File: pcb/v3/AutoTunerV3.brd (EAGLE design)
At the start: 100 x 80 mm, 115 parts, among them IC2 317EMP, Q1 32,768kHz, Q2 BSS123, Q3 BSS84, U1 TPS63070RNMR, Y1 8MHz

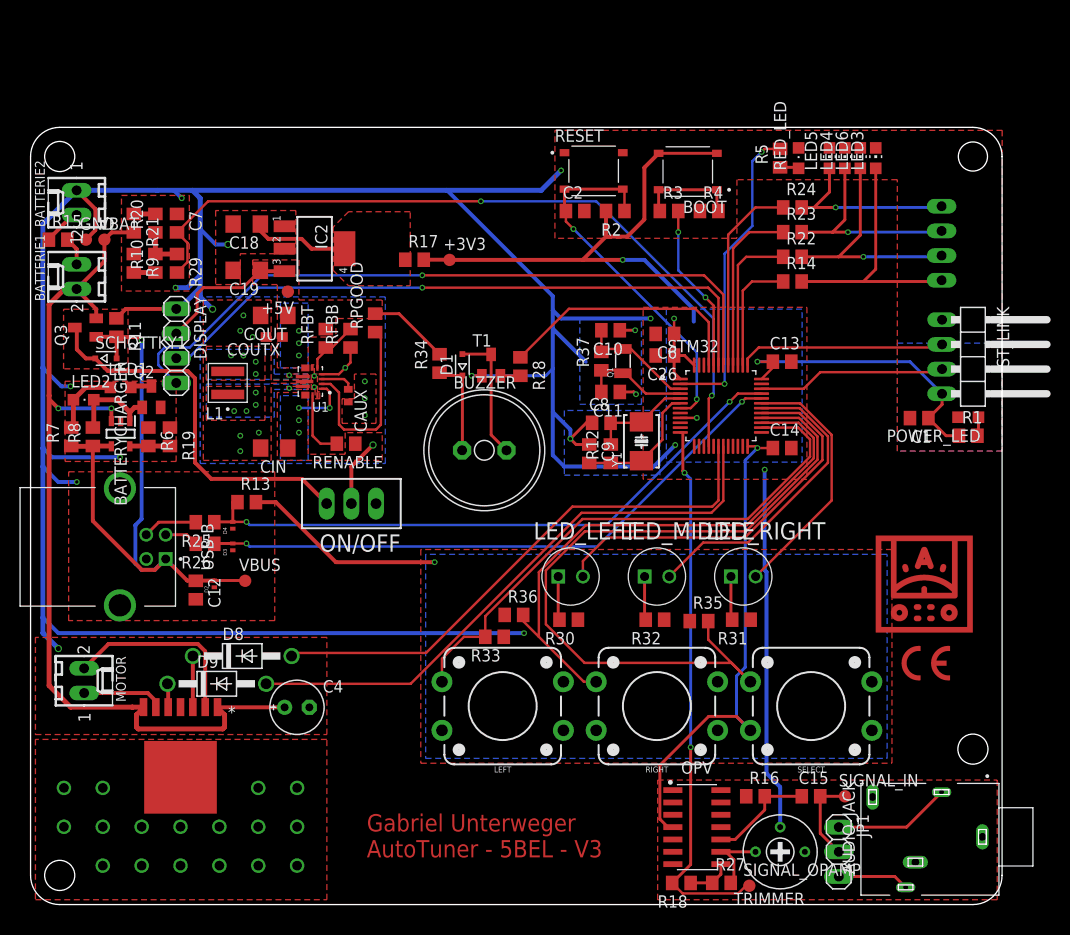
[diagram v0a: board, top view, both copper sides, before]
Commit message: board v3 finished
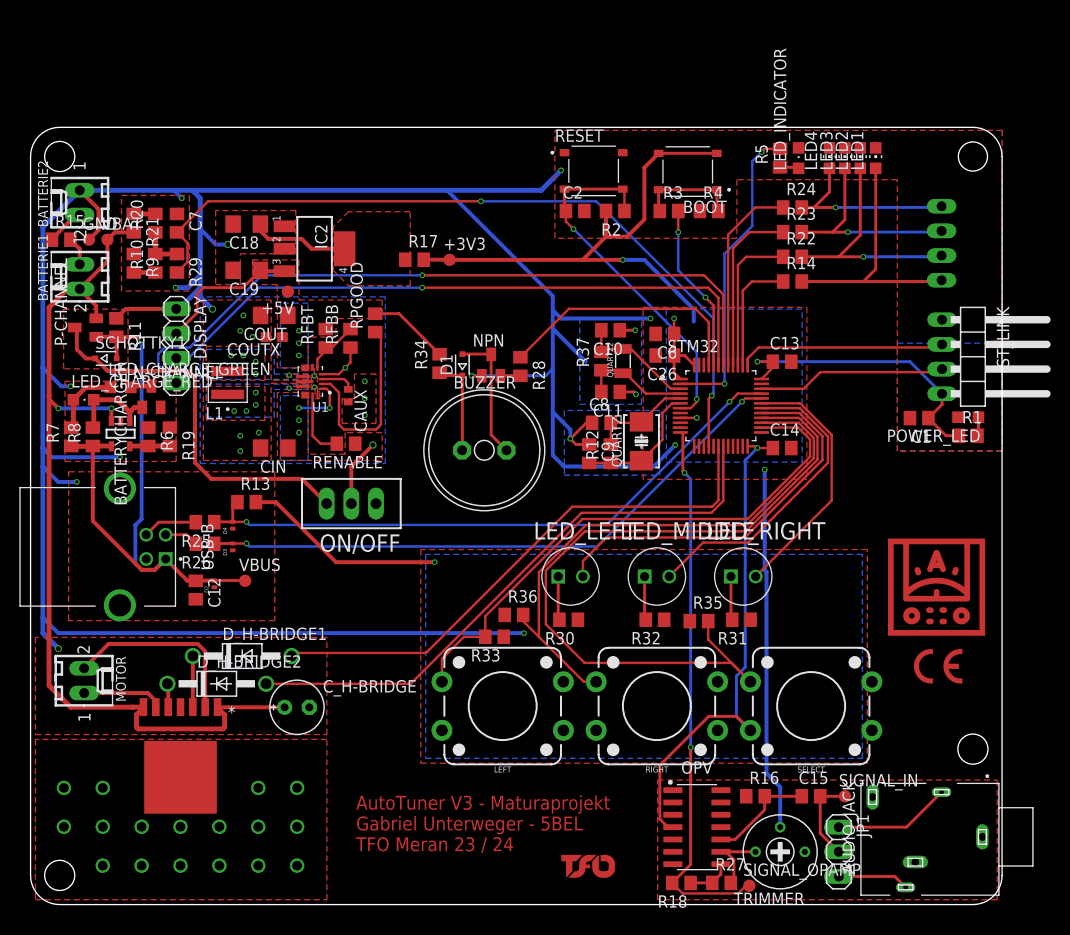
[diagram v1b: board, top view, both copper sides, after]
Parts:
- removed LED5, LED6: (no value), led:CHIP-LED0805
- added LED_CHARGE_GREEN, LED_CHARGE_RED: (no value), led:CHIPLED_0805
- LED1, LED2: device led:CHIPLED_0805 -> led:CHIP-LED0805
- R32: value 60 -> 56
- moved LED2 83.7 mm to (85.4, 76.8), turned to 0 degrees
- moved LED1 81.2 mm to (87.0, 76.8), turned to 0 degrees
- moved LED3 3.18 mm to (83.8, 76.8)
- moved LED4 1.59 mm to (82.2, 76.8)
- moved VBAT 0.32 mm to (7.92, 68.4)
- moved BATTERIE1 0.32 mm to (5.06, 64.6)
- moved BATTERIE2 0.32 mm to (5.06, 72.2)
- moved GND 0.32 mm to (6.01, 68.4)
- moved R15 0.32 mm to (3.15, 68.4)
- renumbered C4 to C_H-BRIDGE, D8 to D_H-BRIDGE1, D9 to D_H-BRIDGE2, JP2 to EXTENSIONS, Q1 to QUARTZ2, Q2 to N-CHANNEL, Q3 to P-CHANNEL, RED_LED to LED_INDICATOR, T1 to NPN, Y1 to QUARTZ
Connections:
- net GND: now also LED1.C, LED2.C; no longer LED5.C, LED6.C
- net N$11: now also LED_CHARGE_GREEN.A, LED_CHARGE_RED.A; no longer LED1.A, LED2.A
- net N$12: now also LED_CHARGE_GREEN.C; no longer LED1.C
- net N$39: now also LED1.A; no longer LED3.A
- net N$48: now also LED2.A; no longer LED6.A
- net N$49: now also LED3.A; no longer LED4.A
- net N$50: now also LED4.A; no longer LED5.A
- net N$9: now also LED_CHARGE_RED.C; no longer LED2.C
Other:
- board text added: "AutoTuner V3 - Maturaprojekt Gabriel Unterweger - 5BEL TFO Meran 23 / 24"
- board text removed: "Gabriel Unterweger AutoTuner - 5BEL - V3"

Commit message: settings menu
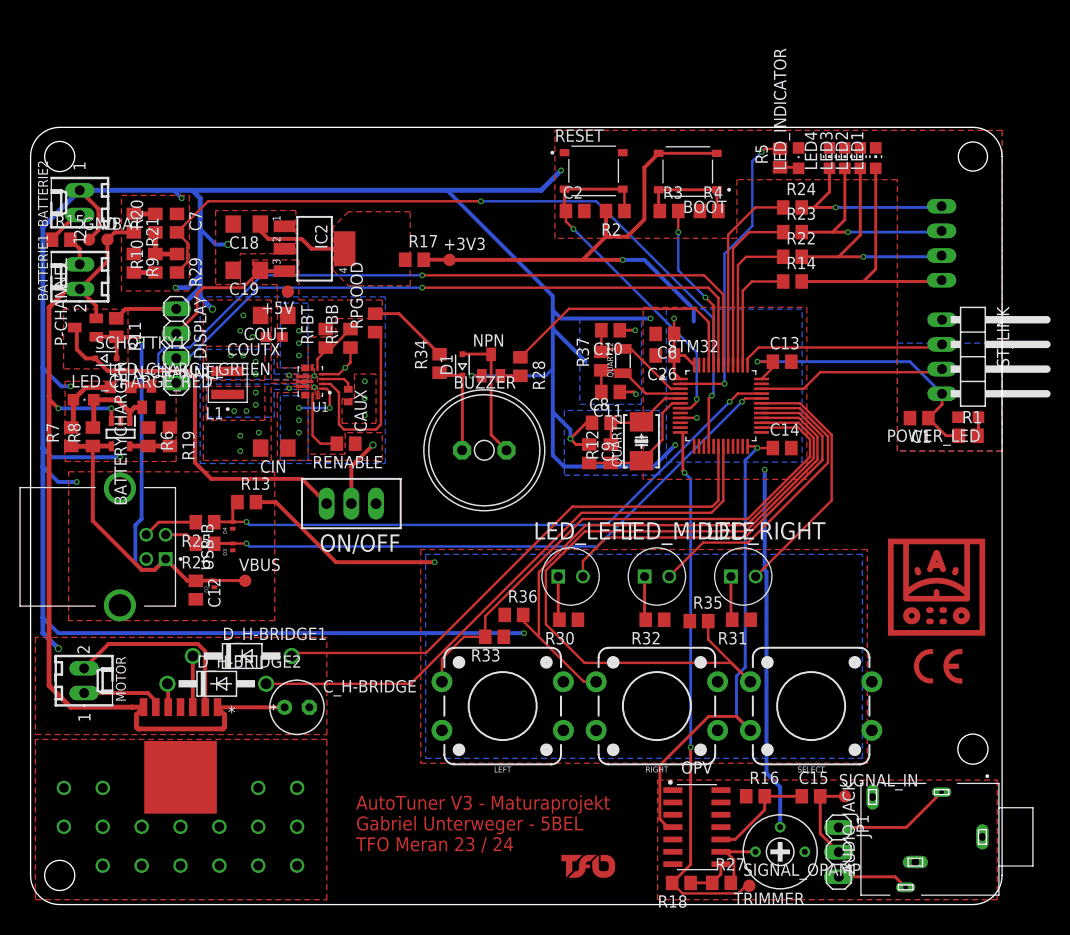
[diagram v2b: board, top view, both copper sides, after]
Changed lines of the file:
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@@
 <drawing>
 <settings>
-<setting alwaysvectorfont="yes"/>
+<setting alwaysvectorfont="no"/>
 <setting verticaltext="up"/>
 </settings>
@@
 <attribute name="VALUE" x="79.675" y="11.035" size="1.27" layer="27" rot="R180"/>
 </element>
-<element name="JP1" library="pinhead" library_urn="urn:adsk.eagle:library:325" package="1X03" package3d_urn="urn:adsk.eagle:package:22458/2" value="" x="83.1925" y="5.43" smashed="yes" rot="R270">
-<attribute name="NAME" x="85.0213" y="9.3162" size="1.27" layer="25" ratio="10" rot="R270"/>
-<attribute name="POPULARITY" value="92" x="83.1925" y="5.43" size="1.778" layer="27" rot="R270" display="off"/>
-<attribute name="VALUE" x="80.0175" y="9.24" size="1.27" layer="27" rot="R270"/>
-</element>
 <element name="LED1" library="led" library_urn="urn:adsk.eagle:library:259" package="CHIP-LED0805" package3d_urn="urn:adsk.eagle:package:15818/2" value="" x="86.995" y="76.835" smashed="yes">
 <attribute name="LCSC_PART" value="C2297" x="86.995" y="76.835" size="1.778" layer="27" display="off"/>
@@
 <attribute name="VALUE" x="25.7175" y="60.325" size="1.27" layer="27" rot="R180"/>
 </element>
+<element name="JP1" library="pinhead" library_urn="urn:adsk.eagle:library:325" package="1X03" package3d_urn="urn:adsk.eagle:package:22458/2" value="" x="83.185" y="5.3975" smashed="yes" rot="R270">
+<attribute name="NAME" x="85.0138" y="9.2837" size="1.27" layer="25" ratio="10" rot="R270"/>
+<attribute name="POPULARITY" value="92" x="83.185" y="5.3975" size="1.778" layer="27" rot="R270" display="off"/>
+<attribute name="VALUE" x="80.01" y="9.2075" size="1.27" layer="27" rot="R270"/>
+</element>
 </elements>
 <signals>
@@
 <signal name="N$11">
 <contactref element="LED_CHARGE_GREEN" pad="A"/>
-<contactref element="LED_CHARGE_RED" pad="A"/>
 <contactref element="R7" pad="2"/>
-<wire x1="4.1875" y1="49.1" x2="4.4075" y2="49.32" width="0.508" layer="1"/>
+<wire x1="8.2175" y1="53.23" x2="5.6775" y2="53.23" width="0.508" layer="1"/>
+<contactref element="LED_CHARGE_RED" pad="A"/>
+<wire x1="5.6775" y1="53.23" x2="4.4075" y2="51.96" width="0.508" layer="1"/>
 <wire x1="4.4075" y1="51.96" x2="4.4075" y2="49.32" width="0.508" layer="1"/>
-<wire x1="4.4075" y1="51.96" x2="5.6775" y2="53.23" width="0.508" layer="1"/>
-<wire x1="5.6775" y1="53.23" x2="8.2175" y2="53.23" width="0.508" layer="1"/>
+<wire x1="4.4075" y1="49.32" x2="4.1875" y2="49.1" width="0.508" layer="1"/>
 </signal>
 <signal name="N$9">
@@
 <contactref element="AUDIO_JACK" pad="5"/>
 <contactref element="JP1" pad="1"/>
-<wire x1="93.775" y1="11.57" x2="90.175" y2="7.97" width="0.3048" layer="1"/>
-<wire x1="90.175" y1="7.97" x2="83.1925" y2="7.97" width="0.3048" layer="1"/>
+<wire x1="90.1425" y1="7.9375" x2="83.185" y2="7.9375" width="0.3048" layer="1"/>
+<wire x1="93.775" y1="11.57" x2="90.1425" y2="7.9375" width="0.3048" layer="1"/>
 </signal>
 <signal name="SIGNAL_IN_2">
 <contactref element="AUDIO_JACK" pad="2"/>
 <contactref element="JP1" pad="3"/>
-<wire x1="83.1925" y1="2.89" x2="88.955" y2="2.89" width="0.3048" layer="1"/>
-<wire x1="88.955" y1="2.89" x2="90.075" y2="1.77" width="0.3048" layer="1"/>
+<wire x1="90.075" y1="1.77" x2="88.9875" y2="2.8575" width="0.3048" layer="1"/>
+<wire x1="88.9875" y1="2.8575" x2="83.185" y2="2.8575" width="0.3048" layer="1"/>
 </signal>
 <signal name="SIGNAL_IN">
-<contactref element="JP1" pad="2"/>
 <contactref element="C15" pad="2"/>
 <contactref element="SIGNAL_IN" pad="TP"/>
-<wire x1="83.1925" y1="5.43" x2="81.285" y2="7.3375" width="0.3048" layer="1"/>
-<wire x1="81.285" y1="7.3375" x2="81.285" y2="11.145" width="0.3048" layer="1"/>
 <wire x1="83.8275" y1="11.145" x2="81.285" y2="11.145" width="0.3048" layer="1"/>
+<contactref element="JP1" pad="2"/>
+<wire x1="83.185" y1="5.3975" x2="81.285" y2="7.2975" width="0.3048" layer="1"/>
+<wire x1="81.285" y1="7.2975" x2="81.285" y2="11.145" width="0.3048" layer="1"/>
 </signal>
 <signal name="CUSTOM2">
